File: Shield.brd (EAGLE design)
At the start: 99.1 x 71.1 mm, 77 parts

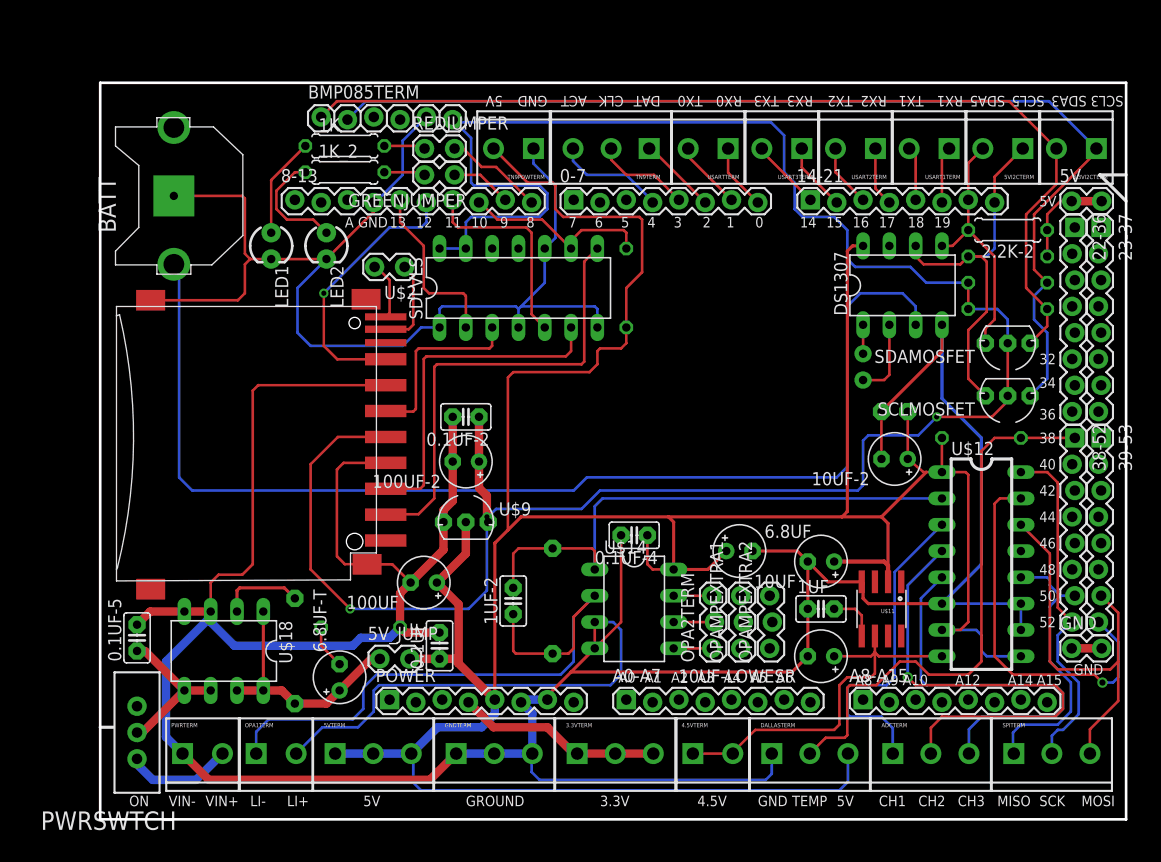
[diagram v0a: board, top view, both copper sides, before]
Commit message: Started Revision 3
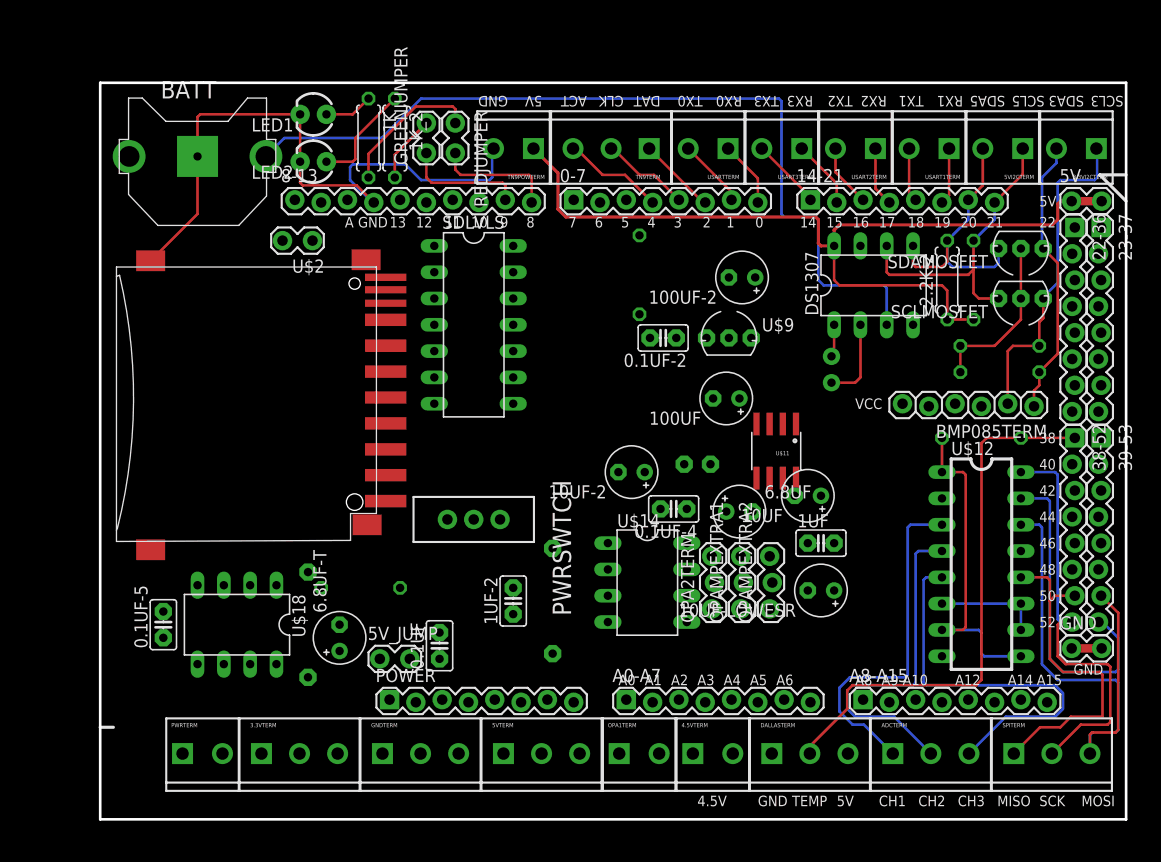
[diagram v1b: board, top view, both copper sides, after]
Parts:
- moved BMP085TERM 62.7 mm to (83.8, 39.9), turned to 180 degrees
- moved PWRSWTCH 38.5 mm to (36.1, 29.0), turned to 270 degrees
- moved OPA1TERM 35.1 mm to (50.3, 6.35)
- moved 100UF 34.2 mm to (60.5, 40.6)
- moved 100UF-2 32.1 mm to (62.0, 52.3)
- moved U$9 31.0 mm to (60.7, 46.5)
- moved 3.3VTERM 30.5 mm to (15.7, 6.35)
- moved 10UF-2 25.4 mm to (51.3, 33.5)
- moved 0.1UF-2 20.5 mm to (54.4, 46.5)
- moved 0.1UF-3 19.7 mm to (57.7, 34.3)
- moved U$11 18.3 mm to (65.3, 35.6)
- moved 5VTERM 16.3 mm to (39.1, 6.35)
- moved LED1 13.3 mm to (20.6, 68.1), turned to 180 degrees
- moved SCLMOSFET 9.48 mm to (88.9, 50.3)
- moved U$2 9.25 mm to (19.1, 55.9)
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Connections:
- net 5V: now also TN9POWTERM.1; no longer TN9POWTERM.2
- net GND: now also TN9POWTERM.2; no longer TN9POWTERM.1
- net VBAT: now also BATT.+2; no longer BATT.+1
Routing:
- net GND: track 487.6 -> 72.3 mm
- net 3.3V: track 218.9 -> 16.3 mm, vias 3 -> 0
- net 5V: track 319.6 -> 118.4 mm
- net 3.3V_SCL: track 103.6 -> 31.7 mm
- net 3.3V_SDA: track 95.1 -> 27.1 mm
- net LIOP-: track 59.6 -> 0.00 mm
- net CH0: track 53.2 -> 0.00 mm
- net SD_CSIN: track 44.3 -> 0.00 mm
- net 4.5V: track 37.5 -> 0.00 mm
- net SD_DATAIN: track 32.8 -> 0.00 mm
- net VBAT: track 111.7 -> 83.2 mm
- net MISO_SOFT: track 26.2 -> 0.00 mm, vias 1 -> 0
- net 5VOUT: track 23.7 -> 0.00 mm
- net MEGA3.3V: track 19.9 -> 0.00 mm
- net MOSI_SOFT: track 19.9 -> 0.00 mm
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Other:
- board text added: "20"
- board text added: "21"
- board text added: "22"
- board text added: "VCC"
- board text removed: "3.3V"
- board text removed: "32"
- board text removed: "34"
- board text removed: "36"
- board text removed: "GROUND"
- board text removed: "LI+"
- board text removed: "LI-"
- board text removed: "ON"
- board text removed: "VIN+"
- board text removed: "VIN-"
